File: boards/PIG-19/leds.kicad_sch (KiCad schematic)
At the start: 4 parts, among them U1 LM2940S-5.0

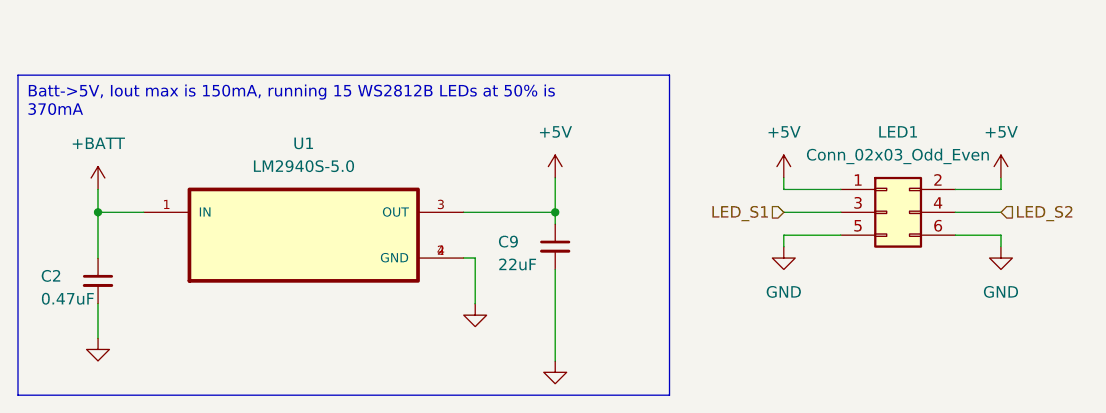
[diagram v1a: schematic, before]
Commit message: board updates
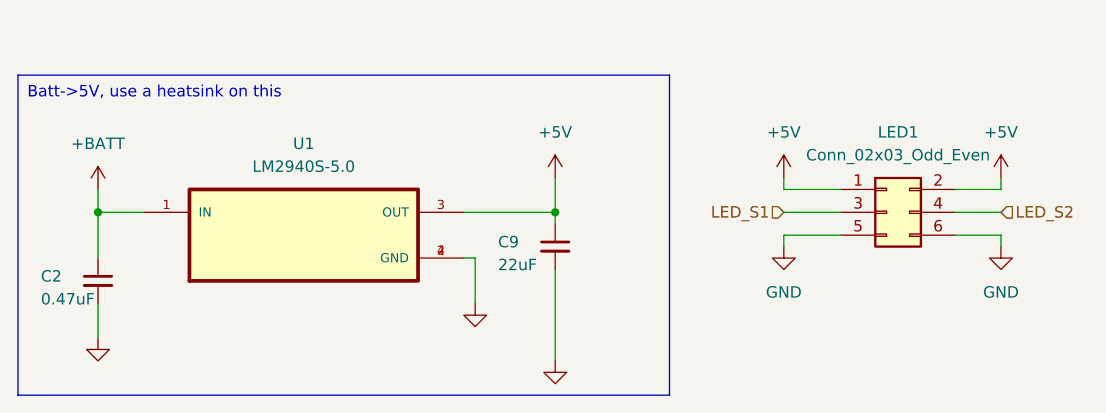
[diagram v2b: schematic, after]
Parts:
- LED1: now left out of the parts list
- U1: MF Texas Instruments -> LM2940S-5.0/NOPB
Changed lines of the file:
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@@
 		)
 	)
-	(text_box "Batt->5V, Iout max is 150mA, running 15 WS2812B LEDs at 50% is 370mA"
+	(text_box "Batt->5V, use a heatsink on this "
 		(exclude_from_sim no)
 		(at 20.32 66.04 0)
@@
 		(unit 1)
 		(exclude_from_sim no)
-		(in_bom yes)
+		(in_bom no)
 		(on_board yes)
 		(dnp no)
@@
 			)
 		)
-		(property "MF" "Texas Instruments"
+		(property "MF" "LM2940S-5.0/NOPB"
 			(at 52.07 83.82 0)
 			(effects
@@
 					(reference "U1")
 					(unit 1)
-				)
-				(path "/469e864f-3700-4a04-a1e1-a9f39f3c0d0e/06412f56-3d2a-46cd-b4d1-06d7ec975c02"
-					(reference "U1")
-					(unit 1)

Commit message: Final Board Revision - pls order this one TAs
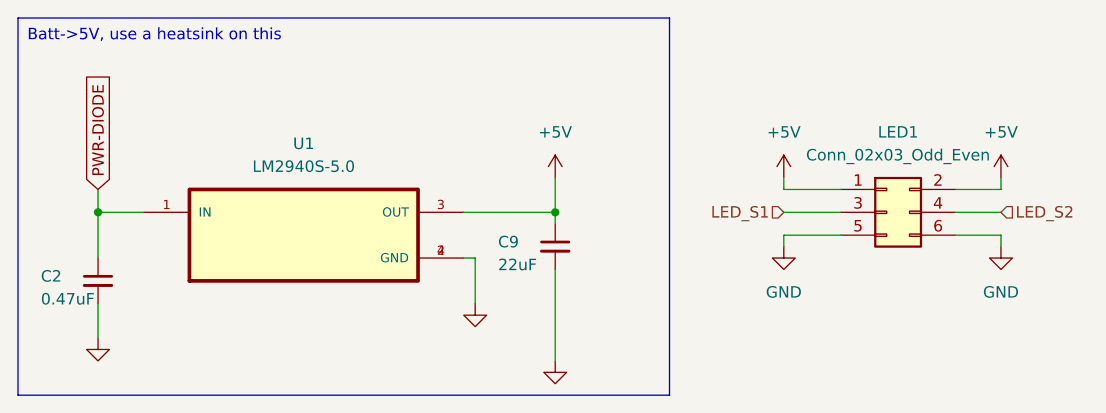
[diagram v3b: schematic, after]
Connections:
- net +BATT renamed PWR-DIODE
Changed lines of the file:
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@@
 	(text_box "Batt->5V, use a heatsink on this "
 		(exclude_from_sim no)
-		(at 20.32 66.04 0)
-		(size 72.39 35.56)
+		(at 20.32 59.69 0)
+		(size 72.39 41.91)
 		(stroke
 			(width 0)
@@
 			)
 			(justify left top)
+		)
+	)
+	(global_label "PWR-DIODE"
+		(shape input)
+		(at 29.21 78.74 90)
+		(fields_autoplaced yes)
+		(effects
+			(font
+				(size 1.27 1.27)
+			)
+			(justify left)
+		)
+		(property "Intersheetrefs" "${INTERSHEET_REFS}"
+			(at 29.21 64.5667 90)
+			(effects
+				(font
+					(size 1.27 1.27)
+				)
+				(justify left)
+				(hide yes)
+			)
 		)
 	)
@@
 					(unit 1)
 				)
-			)
-		)
-	)
-	(symbol
-		(lib_id "power:+BATT")
-		(at 29.21 78.74 0)
-		(unit 1)
-		(exclude_from_sim no)
-		(in_bom yes)
-		(on_board yes)
-		(dnp no)
-		(fields_autoplaced yes)
-		(property "Reference" "#PWR013"
-			(at 29.21 82.55 0)
-			(effects
-				(font
-					(size 1.27 1.27)
-				)
-				(hide yes)
-			)
-		)
-		(property "Value" "+BATT"
-			(at 29.21 73.66 0)
-			(effects
-				(font
-					(size 1.27 1.27)
-				)
-			)
-		)
-		(property "Footprint" ""
-			(at 29.21 78.74 0)
-			(effects
-				(font
-					(size 1.27 1.27)
-				)
-				(hide yes)
-			)
-		)
-		(property "Datasheet" ""
-			(at 29.21 78.74 0)
-			(effects
-				(font
-					(size 1.27 1.27)
-				)
-				(hide yes)
-			)
-		)
-		(property "Description" "Power symbol creates a global label with name \"+BATT\""
-			(at 29.21 78.74 0)
-			(effects
-				(font
-					(size 1.27 1.27)
-				)
-				(hide yes)
-			)
-		)
-		(pin "1"
-		)
-		(instances
-			(project "PIG-19"
-				(path "/469e864f-3700-4a04-a1e1-a9f39f3c0d0e/057bbe4c-afb7-4e9a-9365-c8d142221fbb"
-					(reference "#PWR013")
-					(unit 1)
-				)
